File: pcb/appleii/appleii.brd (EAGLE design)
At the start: 75 x 47 mm, 19 parts, among them J1 POWER_JACKPTH, J2 ATX24RH

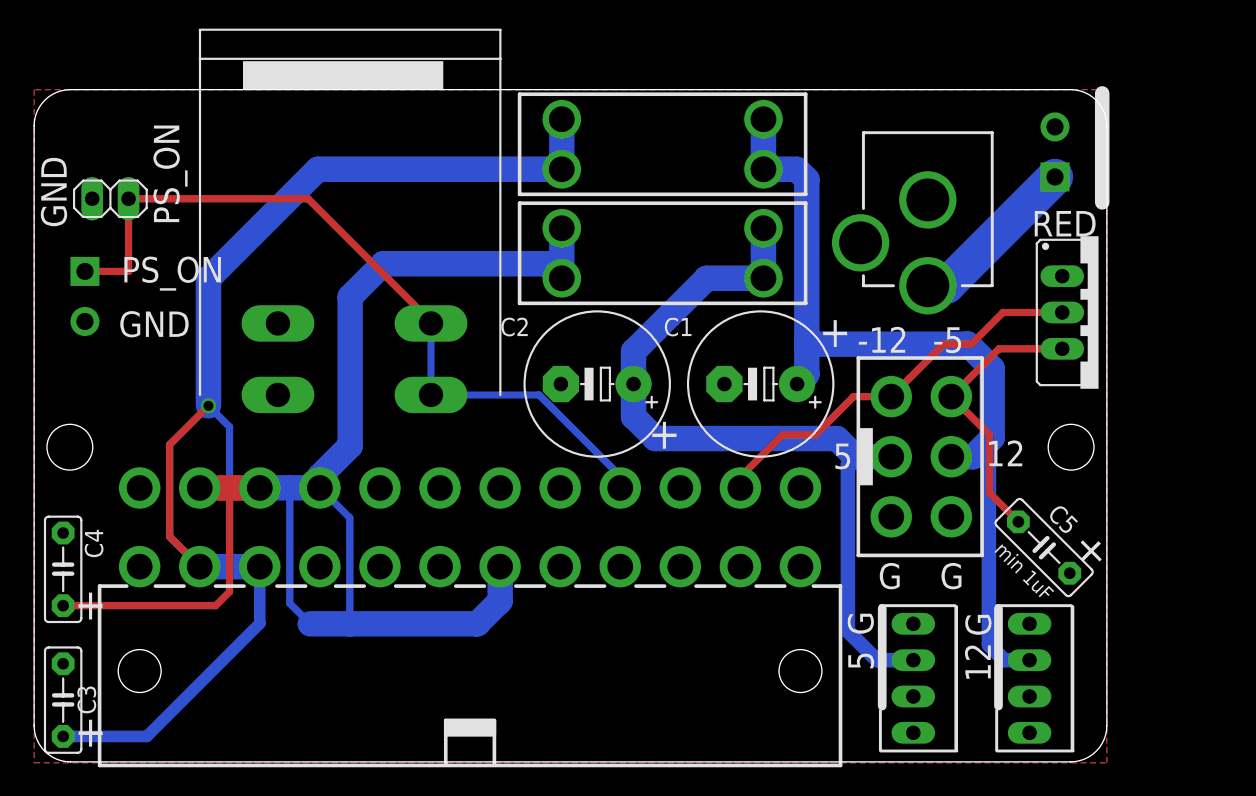
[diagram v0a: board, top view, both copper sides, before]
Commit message: updated pcb
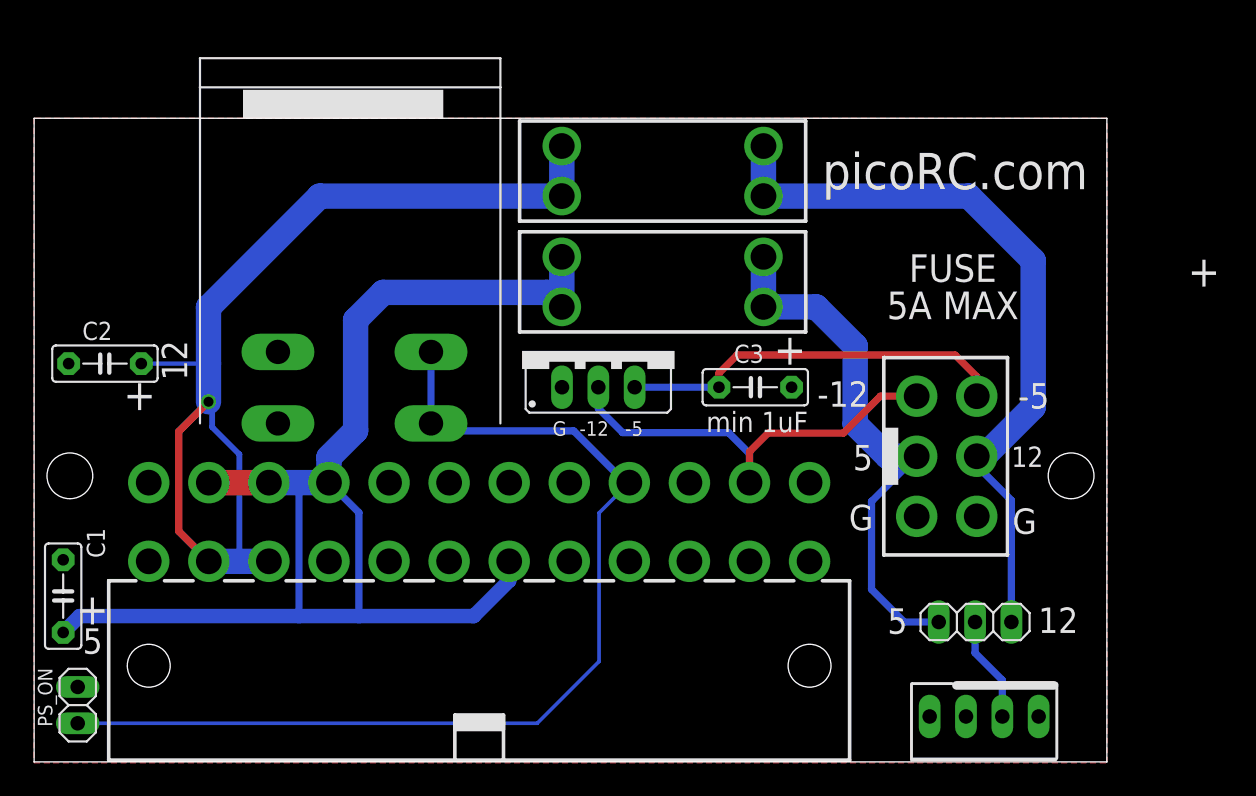
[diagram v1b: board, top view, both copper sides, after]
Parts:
- removed C4, C5: (no value), capacitor-wima:C5B2.5
- removed J2: ATX24RH, macse:ATX24_RIGHT_ANGLE
- removed J3, J7: (no value), atx_power_control:SCREWTERMINAL-3.5MM-2-NS
- removed JP4: (no value), appleii:1X04
- removed U$8: CAR_FUSE_HOLDER3IN1, atx_power_control:FUSE_HOLDER_3IN1
- added JP3: (no value), appleii:1X04
- added U$6: APPLEII, atx4vc:APPLEII
- C1, C2: device rcl:E5-10,5 -> capacitor-wima:C5B2.5
- J1: value POWER_JACKPTH -> ATX24RH; device appleii:POWER_JACK_PTH -> macse:ATX24_RIGHT_ANGLE
- JP1: device appleii:1X04 -> pinhead:1X02
- JP2: device pinhead:1X02 -> pinhead:1X03
- U$1: value M3_MOUNTING_HOLE -> CAR_FUSE_HOLDER3IN1; device a:M3_MOUNTING_HOLE_PACK -> atx_power_control:FUSE_HOLDER_3IN1
- U$3: value M3_MOUNTING_HOLE -> ROCK_SW; device a:M3_MOUNTING_HOLE_PACK -> atx4vc:ROCK_SWITCH
- U$4: value APPLEII -> M3_MOUNTING_HOLE; device atx4vc:APPLEII -> a:M3_MOUNTING_HOLE_PACK
- U$5: value ROCK_SW -> M3_MOUNTING_HOLE; device atx4vc:ROCK_SWITCH -> a:M3_MOUNTING_HOLE_PACK
- moved JP2 67.3 mm to (65.8, 9.78), turned to 0 degrees
- moved JP1 66.6 mm to (3.05, 3.97), turned to 90 degrees
- moved C3 53.1 mm to (50.4, 26.2), turned to 0 degrees
- moved C1 51.0 mm to (2.03, 11.6), turned to 90 degrees
- moved U$3 50.4 mm to (22.1, 23.7)
- moved J1 49.1 mm to (31.1, 9.26), turned to 0 degrees
- moved U$1 43.0 mm to (43.9, 33.6), turned to 180 degrees
- moved IC1 35.1 mm to (39.4, 28.7), turned to 0 degrees
- moved C2 34.4 mm to (4.95, 27.8)
- moved U$5 20.4 mm to (2.50, 20.0)
- moved U$4 10.6 mm to (72.5, 20.0), turned to 0 degrees
- moved U$2 1.87 mm to (43.9, 41.3)
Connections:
- net +12V: now also JP2.3, U$6.4; no longer C1.+, JP1.2, U$4.4
- net +5V: now also JP2.1, U$1.A0, U$1.A1, U$6.3; no longer C2.+, JP4.2, U$4.3, U$8.A0, U$8.A1
- net -12V: now also J1.14, U$6.5; no longer J2.14, U$4.5
- net -5V: now also C3.1, U$6.6; no longer C5.1, U$4.6
- net GND: now also C1.2, C2.2, J1.15, J1.17, J1.18, J1.19, J1.24, J1.3, J1.5, J1.7, JP1.2, JP3.1, U$3.P$1, U$3.P$3, U$6.1, U$6.2; no longer C1.-, C2.-, C4.2, C5.2, J1.GND, J1.GNDBREAK, J2.15, J2.17, J2.18, J2.19, J2.24, J2.3, J2.5, J2.7, J3.2, J7.2, JP1.1, JP2.2, JP4.1, U$4.1, U$4.2, U$5.P$1, U$5.P$3
- net N$1: now also JP2.2, JP3.2; no longer J1.PWR, J3.1
- net N$5: now also J1.16, JP1.1, U$3.P$2, U$3.P$4; no longer J2.16, J7.1, JP2.1, U$5.P$2, U$5.P$4
- net N$6: now also C1.1, J1.21, J1.22, J1.23, J1.6, U$1.B0, U$1.B1; no longer C4.1, J2.21, J2.22, J2.23, J2.6, U$8.B0, U$8.B1
- net N$8: now also C2.1, J1.10, J1.11; no longer C3.1, J2.10, J2.11
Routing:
- net N$8: track 103.8 -> 84.8 mm
- net +5V: track 56.3 -> 38.0 mm
- net N$5: track 54.4 -> 72.2 mm
- net +12V: track 61.2 -> 52.4 mm
- net -5V: track 19.8 -> 27.4 mm
- net N$6: track 98.4 -> 93.2 mm
- net N$1: track 12.0 -> 7.39 mm
- net -12V: track 28.0 -> 30.8 mm
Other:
- board size 75 x 47 mm -> 75 x 45 mm
- board text added: "picoRC.com"
- board text removed: "12V"
- board text removed: "12V Center Positive"
- board text removed: "GND"
- board text removed: "RED"
